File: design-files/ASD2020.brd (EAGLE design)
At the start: 70.5 x 27.5 mm, 11 parts, among them J1 DF12-32-DP, J2 DF12-32-DS, SW1 PTS840 GKP, SW2 PTS840 GKP, U1 ATTINY88-MU

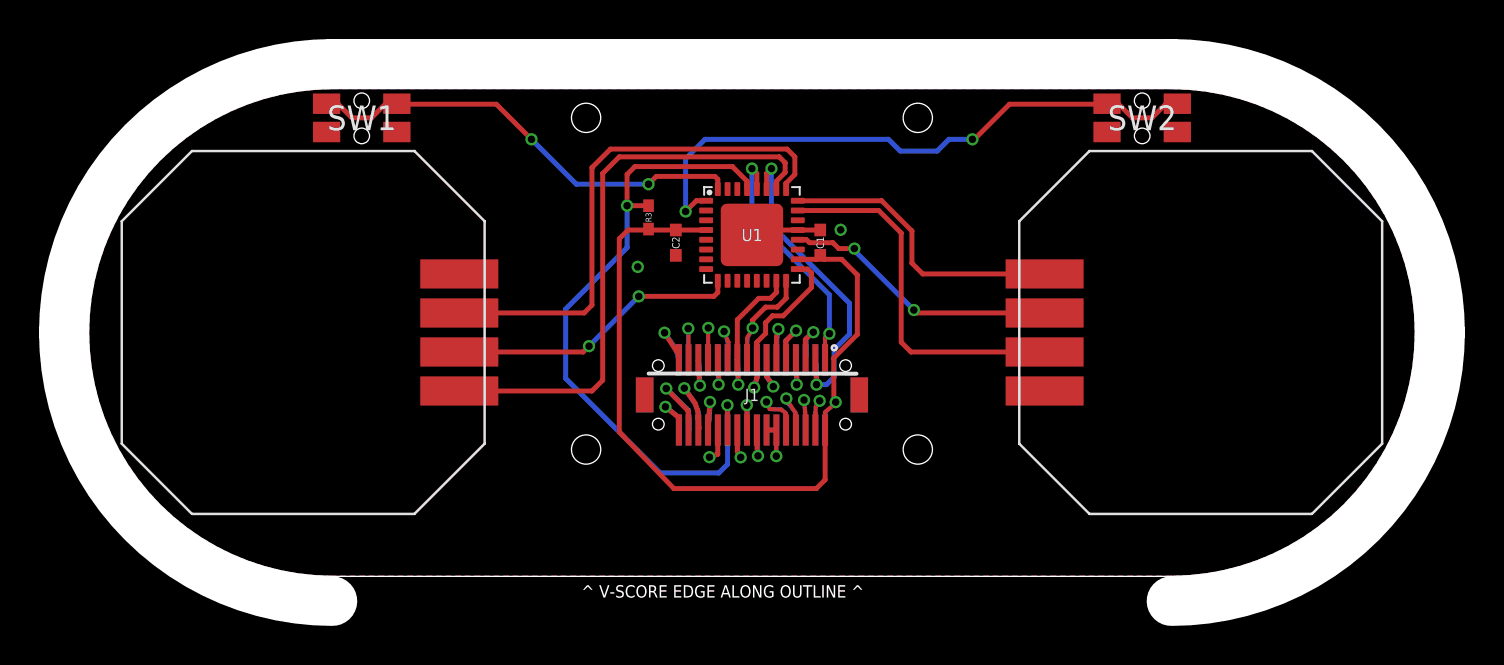
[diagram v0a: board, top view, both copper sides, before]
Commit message: update format
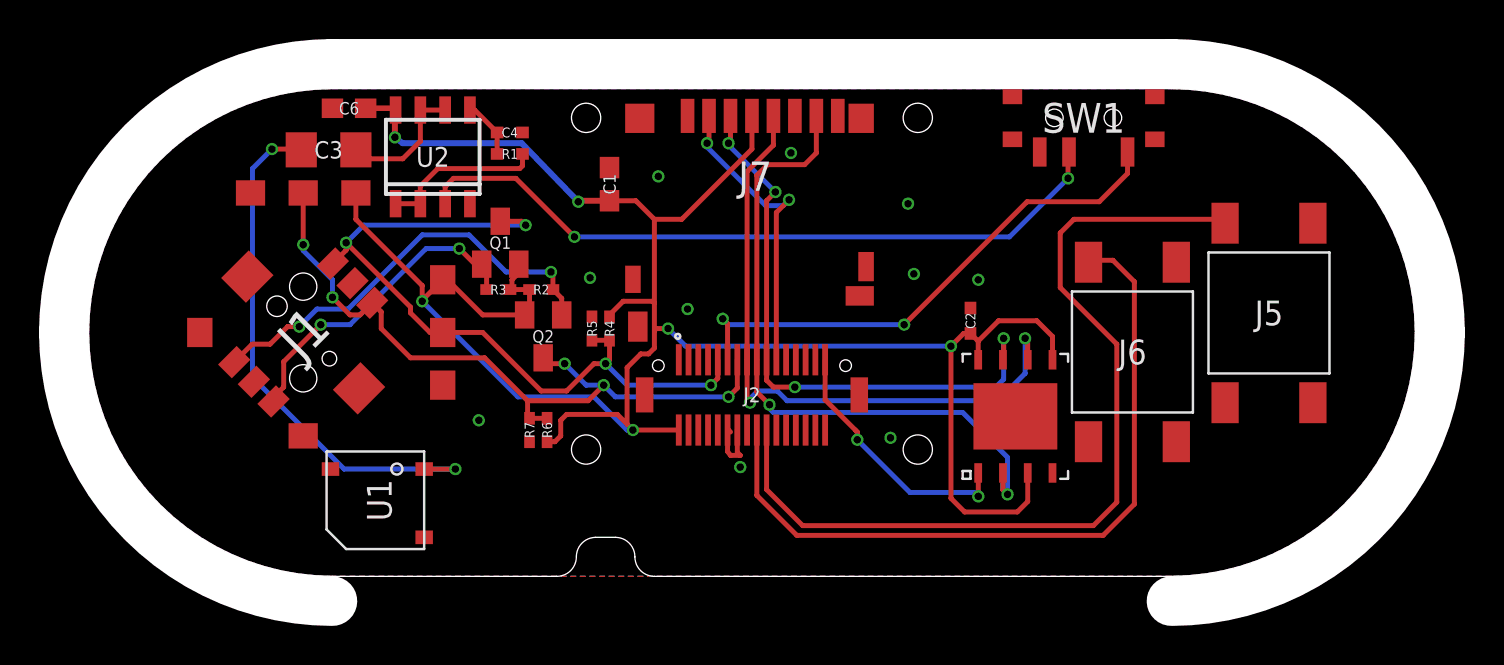
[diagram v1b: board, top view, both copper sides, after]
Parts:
- removed J3, J4: (no value), tinycircuits:PSPJOYSTICK
- removed SW2: PTS840 GKP, tinycircuits:PTS840GKP
- added C3: 100uF, tinycircuits:C1206
- added C4: 10nF, tinycircuits:C0402
- added C6: 10uF, tinycircuits:C0603
- added J5, J6: FSM8JSMA, tinycircuits:SWITCH-FSM/JSM
- added J7: DM3D-SF, tinycircuits:SD_CARD
- added Q1, Q2: DMP2035U, tinycircuits:SOT23
- added R1: 1.00K, tinycircuits:C0402
- added R2, R4, R5, R6, R7: 100K, tinycircuits:0402
- added SW5: 254SA104B50B, tinycircuits:JOYSTICK_CTS_254
- added U2: TS922IDT, tinycircuits:SO-08-COMPACT
- added U3: W25Q64FVZPIG, tinycircuits:8-WSON-6X5
- C1: value 0.1uF -> 10uF; device tinycircuits:C0402 -> tinycircuits:C0603
- J1: value DF12-32-DP -> SKRHABE010; device tinycircuits:DF12-32-DP -> tinycircuits:SKRHA
- R3: value 10.0K -> 100K
- SW1: value PTS840 GKP -> PCM12SMTR; device tinycircuits:PTS840GKP -> tinycircuits:PCM12SMTR
- U1: value ATTINY88-MU -> SMT-0540-S-R; device tinycircuits:ATMEL_QFN32 -> tinycircuits:SMT-0540-S-R
- moved SW1 37.0 mm to (57.0, 28.5)
- moved U1 23.4 mm to (20.9, 8.90), turned to 90 degrees
- moved J1 23.2 mm to (17.0, 17.5), turned to 225 degrees
- moved C2 15.6 mm to (51.2, 18.1), turned to 90 degrees
- moved C1 11.2 mm to (32.7, 25.1)
- moved R3 8.54 mm to (27.0, 19.7), turned to 0 degrees
- flipped J2 to the top
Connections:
- removed net PC0: J4.X, U1.23
- removed net PC1: J4.Y, U1.24
- removed net PC2: J3.X, U1.25
- removed net PC3: J3.Y, U1.26
- removed net PD5: J3.VCC, U1.9
- removed net PD6: J4.VCC, U1.20
- removed net SW0: SW1.3, SW1.4, U1.32
- removed net SW1: SW2.3, SW2.4, U1.1
- new net AUDIOIN: SW1.2, U2.3
- new net N$1: C3.1, U2.6, U2.7
- new net N$12: J1.4, Q1.B, R3.1
- new net N$13: J1.6, Q2.B, R2.1
- new net N$2: C3.2, U1.1
- new net N$4: SW5.S2
- new net N$7: C4.1, R1.2, U2.5
- new net N$9: R1.1, U2.1, U2.2
- new net SW3: SW5.S1
- net +3V3: no longer J1.6
- net +5V: no longer J1.8
- net AD0: now also SW1.1; no longer J1.11
- net AD1: now also J1.3, Q1.C, R4.1, R5.2, SW5.A2; no longer J1.9
- net AD2: no longer J1.7
- net AD3: no longer J1.5
- net AD4/SDA: no longer J1.3, U1.27
- net AD5/SCL: no longer J1.1, U1.28
- net AREF: now also J1.1, Q2.C, R6.1, R7.2, SW5.B2; no longer J1.13
- net GND: now also C4.2, C6.2, J1.5, J5.P$3, J6.P$3, J7.6, R5.1, R7.1, SW1.3, SW5.A1, SW5.B3, U1.2, U2.4, U3.4; no longer J1.12, J1.14, J3.GND, J4.GND, SW1.1, SW1.2, SW2.1, SW2.2, U1.21, U1.5, U1.EXP
- net IO0: no longer J1.24
- net IO1: no longer J1.26
- net IO2: no longer J1.28
- net IO3: no longer J1.30
- net IO4: no longer J1.32
- net IO5: now also U3.1; no longer J1.31
- net IO6: no longer J1.29
- net IO7: no longer J1.27
- net IO8: no longer J1.25
- net IO9: no longer J1.23
- net MISO: now also J7.7, U3.2; no longer J1.17, U1.16
- net MOSI: now also J7.3, U3.7; no longer J1.19, U1.15
- net RESET: no longer J1.22, R3.2, U1.29
- net RSV0: now also J5.P$1; no longer J1.20
- net RSV1: now also J6.P$1; no longer J1.18
- net RSV2: no longer J1.16
- net SCK: now also J7.5, U3.6; no longer J1.15, U1.17
- net SS: now also J7.2; no longer J1.21
- net VBATT: no longer J1.4
- net VCC: now also C6.1, J7.4, Q1.E, Q2.E, R2.2, R3.2, R4.2, R6.2, SW5.A3, SW5.B1, U2.8, U3.3, U3.5, U3.8; no longer J1.2, R3.1, U1.18, U1.4
- net VIN: no longer J1.10
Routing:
- net VCC: track 43.0 -> 118.8 mm, vias 1 -> 6
- net RSV0: track 2.89 -> 46.1 mm, vias 1 -> 0
- net AUDIOIN: track 0.00 -> 36.8 mm, vias 0 -> 2
- net AD1: track 3.42 -> 39.5 mm, vias 1 -> 4
- net RSV1: track 2.56 -> 38.5 mm, vias 1 -> 0
- net AREF: track 2.94 -> 37.7 mm, vias 1 -> 5
- net RESET: track 34.7 -> 0.00 mm, vias 2 -> 0
- net SW1: track 31.4 -> 0.00 mm, vias 2 -> 0
- net PC3: track 29.5 -> 0.00 mm
- net MISO: track 6.88 -> 35.2 mm, vias 1 -> 2
- net N$2: track 0.00 -> 27.6 mm, vias 0 -> 2
- net PC2: track 26.8 -> 0.00 mm
- net AD0: track 3.17 -> 27.4 mm, vias 1 -> 2
- net SCK: track 9.61 -> 33.5 mm, vias 1 -> 2
- net SW0: track 23.1 -> 0.00 mm, vias 2 -> 0
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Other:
- outline, holes or cut-outs redrawn
- board text added: "4"
- board text added: "ASD2020 - Rev4"
- board text added: "TinyCircuits.com"
- board text removed: "3"
- board text removed: "ASD2020 - Rev3"
- board text removed: "Tiny-Circuits.com"
